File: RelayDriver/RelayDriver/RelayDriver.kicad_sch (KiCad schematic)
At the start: 16 parts, among them J1 USB_B_Micro, U1 FT4222HQ, U2 DRV81008Q, U3 DRV81008Q, U4 DRV81008Q, Y1 SG-210STF

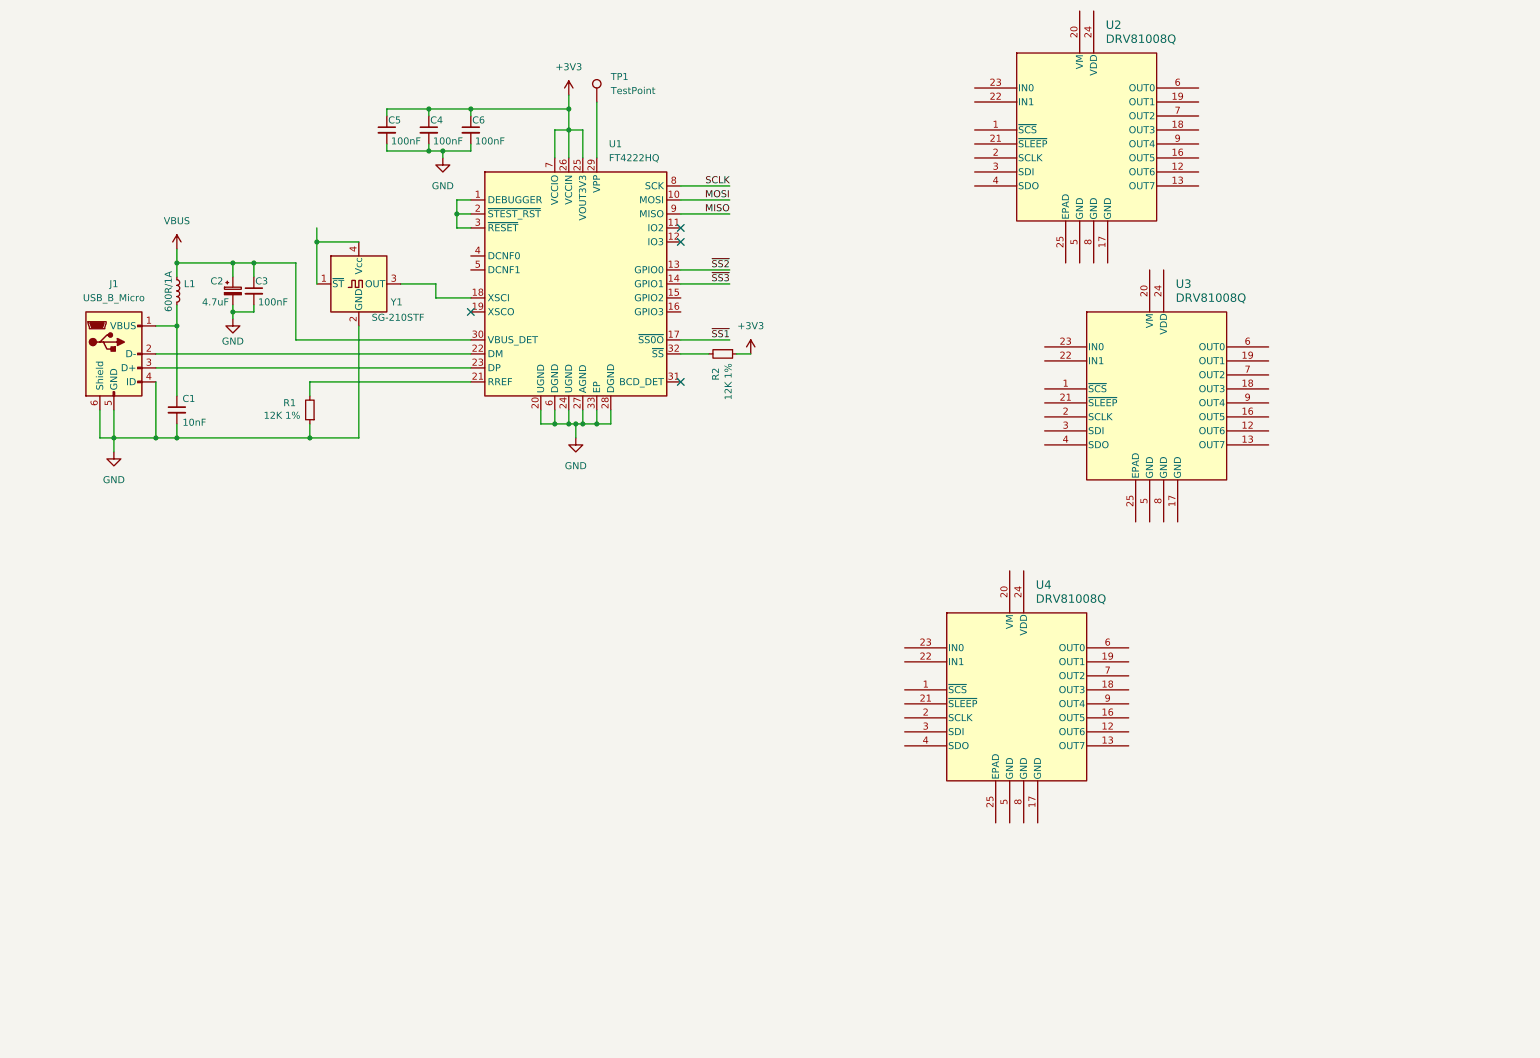
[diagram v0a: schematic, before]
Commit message: Continue editing Rev A
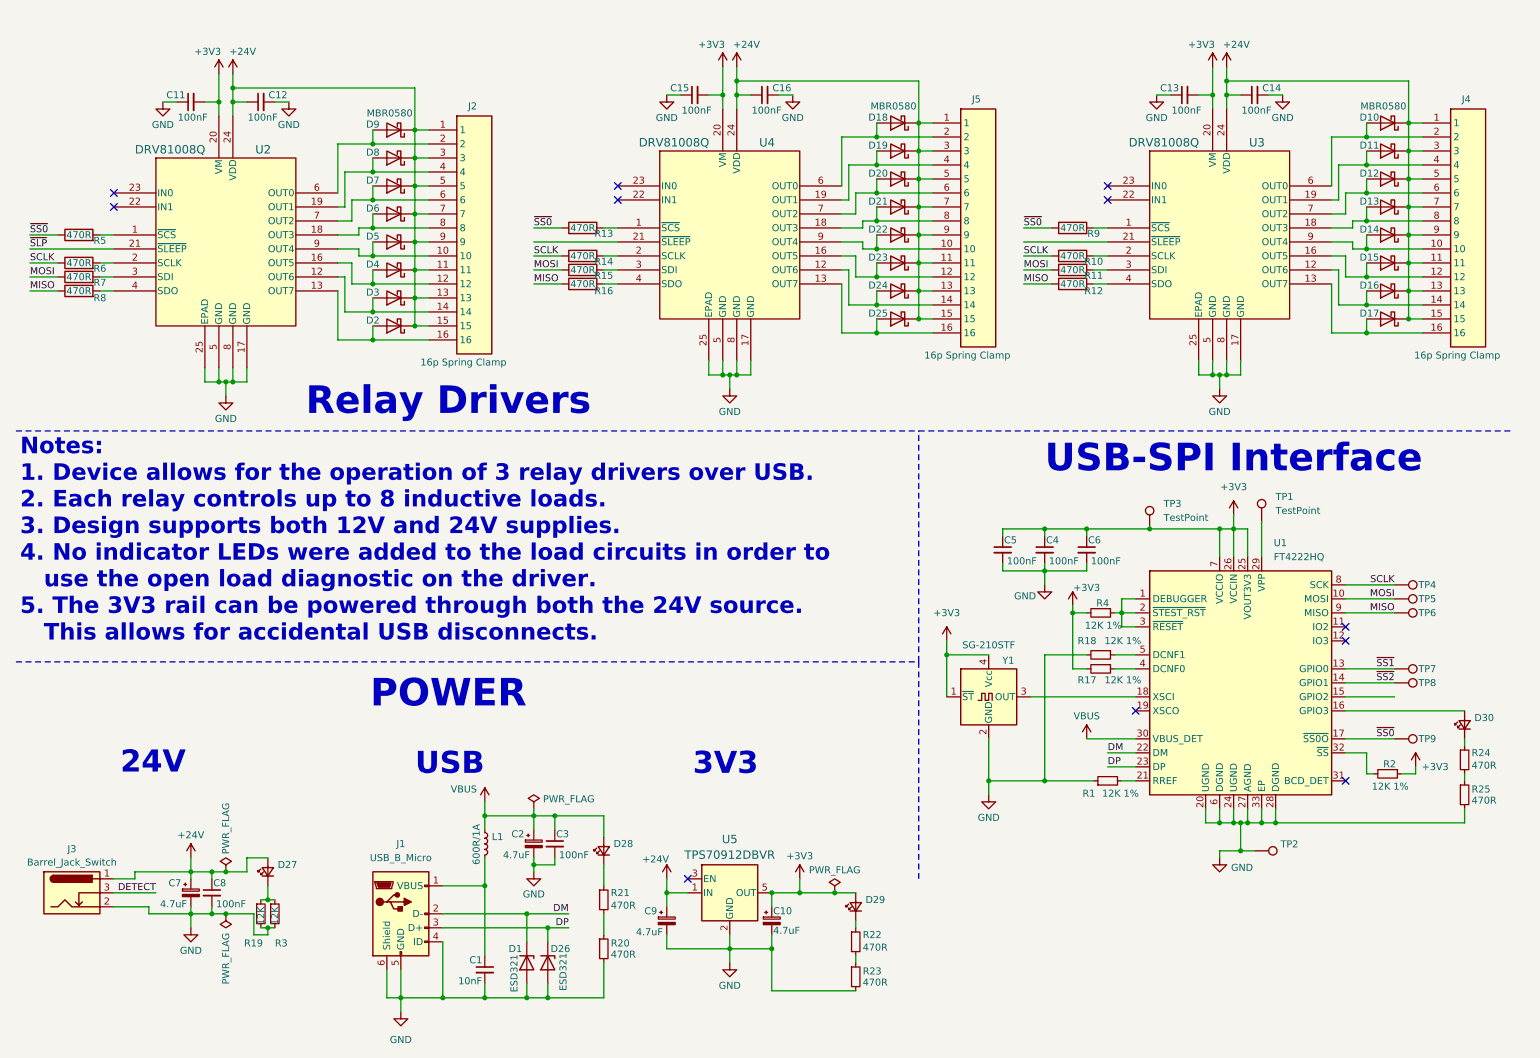
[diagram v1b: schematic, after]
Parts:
- added C10, C7, C9: 4.7uF, symbol Device:C_Polarized_Small
- added C11, C12, C13, C14, C15, C16, C8: 100nF, symbol Device:C_Small
- added D1, D26: ESD321, Diode_SMD:D_SOD-523, symbol Diode:ESD5Zxx
- added D10, D11, D12, D13, D14, D15, D16, D17, D18, D19, D2, D20, D21, D22, D23, D24, D25, D3, D4, D5, D6, D7, D8, D9: MBR0580, Diode_SMD:D_SOD-123, symbol Diode:MBR0580
- added D27, D28, D29, D30: LED_Small, symbol Device:LED_Small
- added J2, J4, J5: 16p Spring Clamp, Custom:1989887, symbol custom-components:Phoenix 1989887
- added J3: Barrel_Jack_Switch, symbol Connector:Barrel_Jack_Switch
- added R10, R11, R12, R13, R14, R15, R16, R5, R6, R7, R8, R9: 470R, symbol Device:R
- added R17, R18, R4: 12K 1%, symbol Device:R_Small
- added R19, R3: 12K, symbol Device:R_Small
- added R20, R21, R22, R23, R24, R25: 470R, symbol Device:R_Small
- added TP2, TP3, TP4, TP5, TP6, TP7, TP8, TP9: TestPoint, MountingHole:MountingHole_3.2mm_M3_DIN965_Pad, symbol Connector:TestPoint
- added U5: TPS70912DBVR, Custom:DBV5_TEX, symbol custom-components:TPS70912DBVR
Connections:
- net ~{SS3} is gone; now on net ~{SS2}: U1.14 (GPIO1)
- net +3V3: now also U2.20 (VM), U3.20 (VM), U4.20 (VM), Y1.1 (~{ST}), Y1.4 (Vcc), C10.1, C11.2, C13.2, C15.2, D29.2 (A), R17.2, R4.2, TP3.1, U5.5 (OUT)
- net GND: now also U2.17 (GND), U2.25 (EPAD), U2.5 (GND), U2.8 (GND), U3.17 (GND), U3.25 (EPAD), U3.5 (GND), U3.8 (GND), U4.17 (GND), U4.25 (EPAD), U4.5 (GND), U4.8 (GND), C10.2, C11.1, C12.2, C13.1, C14.2, C15.1, C16.2, C7.2, C8.2, C9.2, D1.2 (A), D26.2 (A), J3.2, R18.2, R19.2, R20.2, R23.2, R25.2, R3.2, TP2.1, U5.2 (GND)
- net MISO: now also R12.1, R16.1, R8.1, TP6.1
- net MOSI: now also R11.1, R15.1, R7.1, TP5.1
- net SCLK: now also R10.1, R14.1, R6.1, TP4.1
- net VBUS: now also D28.2 (A)
- net ~{SS1}: now also U1.13 (GPIO0), TP7.1; no longer U1.17 (~{SS0O})
- net ~{SS2}: now also TP8.1; no longer U1.13 (GPIO0)
- net at U2.1 (~{SCS}): now also R5.2
- net at U2.12 (OUT6): now also D3.2 (A), J2.14
- net at U2.13 (OUT7): now also D2.2 (A), J2.16
- net at U2.16 (OUT5): now also D4.2 (A), J2.12
- net at U2.18 (OUT3): now also D6.2 (A), J2.8
- net at U2.19 (OUT1): now also D8.2 (A), J2.4
- net at U2.2 (SCLK): now also R6.2
- net ~{SLP}: now reaches U2.21 (~{SLEEP})
- net +24V: now reaches U2.24 (VDD)
- net +24V: now also U3.24 (VDD), U4.24 (VDD), C12.1, C14.1, C16.1, C7.1, C8.1, C9.1, D10.1 (K), D11.1 (K), D12.1 (K), D13.1 (K), D14.1 (K), D15.1 (K), D16.1 (K), D17.1 (K), D18.1 (K), D19.1 (K), D2.1 (K), D20.1 (K), D21.1 (K), D22.1 (K), D23.1 (K), D24.1 (K), D25.1 (K), D27.2 (A), D3.1 (K), D4.1 (K), D5.1 (K), D6.1 (K), D7.1 (K), D8.1 (K), D9.1 (K), J2.1, J2.11, J2.13, J2.15, J2.3, J2.5, J2.7, J2.9, J3.1, J4.1, J4.11, J4.13, J4.15, J4.3, J4.5, J4.7, J4.9, J5.1, J5.11, J5.13, J5.15, J5.3, J5.5, J5.7, J5.9, U5.1 (IN)
- net at U2.3 (SDI): now also R7.2
- net at U2.4 (SDO): now also R8.2
- net at U2.6 (OUT0): now also D9.2 (A), J2.2
- net at U2.7 (OUT2): now also D7.2 (A), J2.6
- net at U2.9 (OUT4): now also D5.2 (A), J2.10
- net at U3.1 (~{SCS}): now also R9.2
- net at U3.12 (OUT6): now also D16.2 (A), J4.14
- net at U3.13 (OUT7): now also D17.2 (A), J4.16
- net at U3.16 (OUT5): now also D15.2 (A), J4.12
- net at U3.18 (OUT3): now also D13.2 (A), J4.8
- net at U3.19 (OUT1): now also D11.2 (A), J4.4
- net at U3.2 (SCLK): now also R10.2
- net at U3.3 (SDI): now also R11.2
- net at U3.4 (SDO): now also R12.2
- net at U3.6 (OUT0): now also D10.2 (A), J4.2
- net at U3.7 (OUT2): now also D12.2 (A), J4.6
- net at U3.9 (OUT4): now also D14.2 (A), J4.10
- net at U4.1 (~{SCS}): now also R13.2
- net at U4.12 (OUT6): now also D24.2 (A), J5.14
- net at U4.13 (OUT7): now also D25.2 (A), J5.16
- net at U4.16 (OUT5): now also D23.2 (A), J5.12
- net at U4.18 (OUT3): now also D21.2 (A), J5.8
- net at U4.19 (OUT1): now also D19.2 (A), J5.4
- net at U4.2 (SCLK): now also R14.2
- net at U4.3 (SDI): now also R15.2
- net at U4.4 (SDO): now also R16.2
- net at U4.6 (OUT0): now also D18.2 (A), J5.2
- net at U4.7 (OUT2): now also D20.2 (A), J5.6
- net at U4.9 (OUT4): now also D22.2 (A), J5.10
- net DM: now reaches J1.2 (D-), U1.22 (DM)
- net DM: now also D1.1 (K)
- net DP: now reaches J1.3 (D+), U1.23 (DP)
- net DP: now also D26.1 (K)
- net at U1.1 (DEBUGGER), U1.2 (~{STEST_RST}), U1.3 (~{RESET}): now also R4.1
- net at U1.16 (GPIO3): now also D30.2 (A)
- net at U1.4 (DCNF0): now also R17.1
- net at U1.5 (DCNF1): now also R18.1
- new net: R24.2, R25.1
- new net: R20.1, R21.2
- new net: D28.1 (K), R21.1
- new net: R22.2, R23.1
- new net: D27.1 (K), R19.1, R3.1
- new net: D30.1 (K), R24.1
- new net: D29.1 (K), R22.1
- new net DETECT: J3.3
- new net ~{SS0}: R13.1, R5.1, R9.1, TP9.1, U1.17 (~{SS0O})
- no-connect marks 4 -> 11
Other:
- note added: "24V"
- note added: "3V3"
- note added: "Notes: 1. Device allows for the operation of 3 relay drivers over USB. 2. Each relay controls up to 8 inductive loads. 3. Design supports both 12V and 24V supplies. 4. No indicator LEDs were added to the load circuits in order to use the open load diagnostic on the driver. 5. The 3V3 rail can be powered through both the 24V source. This allows for accidental USB disconnects."
- note added: "POWER"
- note added: "Relay Drivers"
- note added: "USB"
- note added: "USB-SPI Interface"
- moved on the sheet: C1, C2, C3, C4, C5, C6, J1, L1, R1, R2, TP1, U1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
